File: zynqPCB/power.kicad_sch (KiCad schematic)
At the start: 60 parts, among them CON1 AVR-JTAG-10, U10 SC189 - 3.3V, U11 TLV62080DSGx, U12 SC189 - 1.8V, U2 SN74AUP1G32DPWR, U20 xc7z020clg484, U3 SN74LVC1G08DSFR, U7 LM3880, U8 LM3880, U9 SC189 - 1.0V

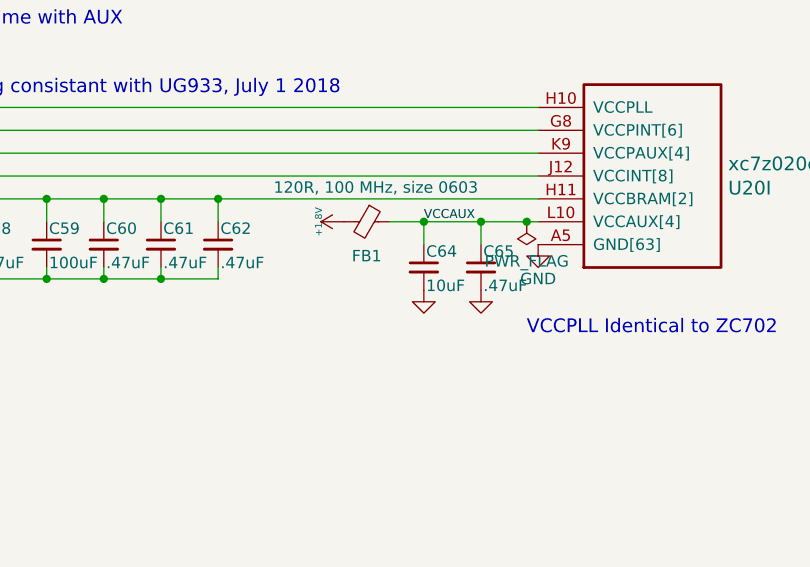
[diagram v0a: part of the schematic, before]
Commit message: Ferrite Bead
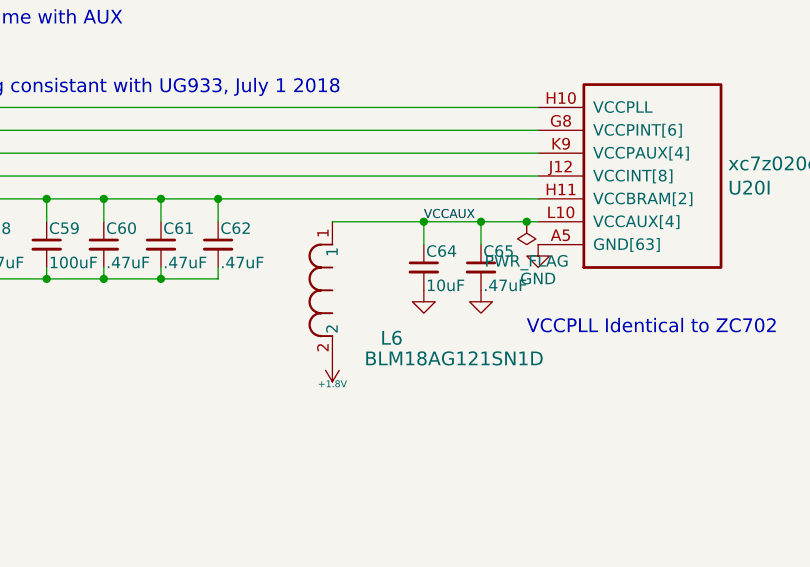
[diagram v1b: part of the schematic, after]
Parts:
- removed FB1: 120R, 100 MHz, size 0603, Inductor_SMD:L_0603_1608Metric, symbol Device:Ferrite_Bead_Small
- added L6: BLM18AG121SN1D, DFTcustom:IND_BLM18_0603_MUR-L, symbol Ferrite_Bead:BLM18AG121SN1D
- U2: footprint Or_gate:DPW0005A_TEX -> DFTcustom:DPW0005A_TEX
- U3: footprint SINGLE_AND_GATE:SON35P100X100X40-6N -> DFTcustom:SON35P100X100X40-6N
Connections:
- net +1.8V: now also L6.2
- net VCCAUX: now also L6.1
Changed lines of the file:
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@@
 	(wire
 		(pts
+			(xy 234.95 160.02) (xy 245.11 160.02)
+		)
+		(stroke
+			(width 0)
+			(type default)
+		)
+	)
+	(wire
+		(pts
 			(xy 76.2 186.69) (xy 76.2 175.26)
 		)
@@
 	(wire
 		(pts
-			(xy 241.3 160.02) (xy 245.11 160.02)
-		)
-		(stroke
-			(width 0)
-			(type default)
-		)
-	)
-	(wire
-		(pts
 			(xy 99.06 86.36) (xy 114.3 86.36)
 		)
@@
 	)
 	(symbol
-		(lib_id "Device:Ferrite_Bead_Small")
-		(at 238.76 160.02 270)
-		(unit 1)
-		(body_style 1)
-		(exclude_from_sim no)
-		(in_bom yes)
-		(on_board yes)
-		(in_pos_files yes)
-		(dnp no)
-		(property "Reference" "FB1"
-			(at 238.76 163.83 90)
-			(show_name no)
-			(do_not_autoplace no)
-			(effects
-				(font
-					(size 1.27 1.27)
-				)
-			)
-		)
-		(property "Value" "120R, 100 MHz, size 0603"
-			(at 239.776 156.21 90)
-			(show_name no)
-			(do_not_autoplace no)
-			(effects
-				(font
-					(size 1.27 1.27)
-				)
-			)
-		)
-		(property "Footprint" "Inductor_SMD:L_0603_1608Metric"
-			(at 238.76 158.242 90)
-			(hide yes)
-			(show_name no)
-			(do_not_autoplace no)
-			(effects
-				(font
-					(size 1.27 1.27)
-				)
-			)
-		)
-		(property "Datasheet" ""
-			(at 238.76 160.02 0)
-			(hide yes)
-			(show_name no)
-			(do_not_autoplace no)
-			(effects
-				(font
-					(size 1.27 1.27)
-				)
-			)
-		)
-		(property "Description" ""
-			(at 238.76 160.02 0)
-			(show_name no)
-			(do_not_autoplace no)
-			(effects
-				(font
-					(size 1.27 1.27)
-				)
-			)
-		)
-		(property "MFR" "Murata Electronics"
-			(at 78.74 -78.74 0)
-			(hide yes)
-			(show_name no)
-			(do_not_autoplace no)
-			(effects
-				(font
-					(size 1.27 1.27)
-				)
-			)
-		)
-		(property "MPN" "BLM18AG121SN1D"
-			(at 78.74 -78.74 0)
-			(hide yes)
-			(show_name no)
-			(do_not_autoplace no)
-			(effects
-				(font
-					(size 1.27 1.27)
-				)
-			)
-		)
-		(property "SPR" "Digikey"
-			(at 78.74 -78.74 0)
-			(hide yes)
-			(show_name no)
-			(do_not_autoplace no)
-			(effects
-				(font
-					(size 1.27 1.27)
-				)
-			)
-		)
-		(property "SPN" "490-1011-1-ND"
-			(at 78.74 -78.74 0)
-			(hide yes)
-			(show_name no)
-			(do_not_autoplace no)
-			(effects
-				(font
-					(size 1.27 1.27)
-				)
-			)
-		)
-		(property "SPURL" "-"
-			(at 78.74 -78.74 0)
-			(hide yes)
-			(show_name no)
-			(do_not_autoplace no)
-			(effects
-				(font
-					(size 1.27 1.27)
-				)
-			)
-		)
-		(pin "1"
-		)
-		(pin "2"
-		)
-		(instances
-			(project "DFTBoard"
-				(path "/49eba173-d38c-4d05-b21c-b4a14c4948c2/00000000-0000-0000-0000-000058508414"
-					(reference "FB1")
-					(unit 1)
-				)
-			)
-		)
-	)
-	(symbol
 		(lib_id "power:+1V8")
-		(at 236.22 160.02 90)
+		(at 234.95 175.26 180)
 		(unit 1)
 		(body_style 1)
@@
 		(dnp no)
 		(property "Reference" "#PWR0110"
-			(at 232.664 160.02 0)
+			(at 234.95 178.816 0)
 			(hide yes)
 			(show_name no)
@@
 		)
 		(property "Value" "+1.8V"
-			(at 233.426 160.02 0)
+			(at 234.95 178.054 0)
 			(show_name no)
 			(do_not_autoplace no)
@@
 		)
 		(property "Footprint" ""
-			(at 236.22 160.02 0)
+			(at 234.95 175.26 0)
 			(hide yes)
 			(show_name no)
@@
 		)
 		(property "Datasheet" ""
-			(at 236.22 160.02 0)
+			(at 234.95 175.26 0)
 			(hide yes)
 			(show_name no)
@@
 		)
 		(property "Description" ""
-			(at 236.22 160.02 0)
+			(at 234.95 175.26 0)
 			(show_name no)
 			(do_not_autoplace no)
@@
 			)
 		)
-		(property "Footprint" "Or_gate:DPW0005A_TEX"
+		(property "Footprint" "DFTcustom:DPW0005A_TEX"
 			(at 17.78 171.45 0)
 			(hide yes)
@@
 	)
 	(symbol
+		(lib_id "Ferrite_Bead:BLM18AG121SN1D")
+		(at 234.95 175.26 90)
+		(unit 1)
+		(body_style 1)
+		(exclude_from_sim no)
+		(in_bom yes)
+		(on_board yes)
+		(in_pos_files yes)
+		(dnp no)
+		(property "Reference" "L6"
+			(at 240.284 172.974 90)
+			(show_name no)
+			(do_not_autoplace no)
+			(effects
+				(font
+					(size 1.524 1.524)
+				)
+				(justify right)
+			)
+		)
+		(property "Value" "BLM18AG121SN1D"
+			(at 238.506 175.26 90)
+			(show_name no)
+			(do_not_autoplace no)
+			(effects
+				(font
+					(size 1.524 1.524)
+				)
+				(justify right)
+			)
+		)
+		(property "Footprint" "DFTcustom:IND_BLM18_0603_MUR-L"
+			(at 234.95 175.26 0)
+			(hide yes)
+			(show_name no)
+			(do_not_autoplace no)
+			(effects
+				(font
+					(size 1.27 1.27)
+					(italic yes)
+				)
+			)
+		)
+		(property "Datasheet" "BLM18AG121SN1D"
+			(at 234.95 175.26 0)
+			(hide yes)
+			(show_name no)
+			(do_not_autoplace no)
+			(effects
+				(font
+					(size 1.27 1.27)
+					(italic yes)
+				)
+			)
+		)
+		(property "Description" ""
+			(at 234.95 175.26 0)
+			(hide yes)
+			(show_name no)
+			(do_not_autoplace no)
+			(effects
+				(font
+					(size 1.27 1.27)
+				)
+			)
+		)
+		(pin "1"
+		)
+		(pin "2"
+		)
+		(instances
+			(project "DFTBoard"
+				(path "/49eba173-d38c-4d05-b21c-b4a14c4948c2/00000000-0000-0000-0000-000058508414"
+					(reference "L6")
+					(unit 1)
+				)
+			)
+		)
+	)
+	(symbol
 		(lib_id "power:+5V")
 		(at 110.49 177.8 0)
@@
 			)
 		)
-		(property "Footprint" "SINGLE_AND_GATE:SON35P100X100X40-6N"
+		(property "Footprint" "DFTcustom:SON35P100X100X40-6N"
 			(at 12.7 190.5 0)
 			(hide yes)
